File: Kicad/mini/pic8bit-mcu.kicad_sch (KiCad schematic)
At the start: 29 parts, among them IC201 TLV1117-33, IC202 MICROCHIP-PIC16F1778-ISP, K201 *Power & UART, K202 MCU 1, K203 MCU 1, K204 ICSP, K205 MCU 2, K206 MCU 2

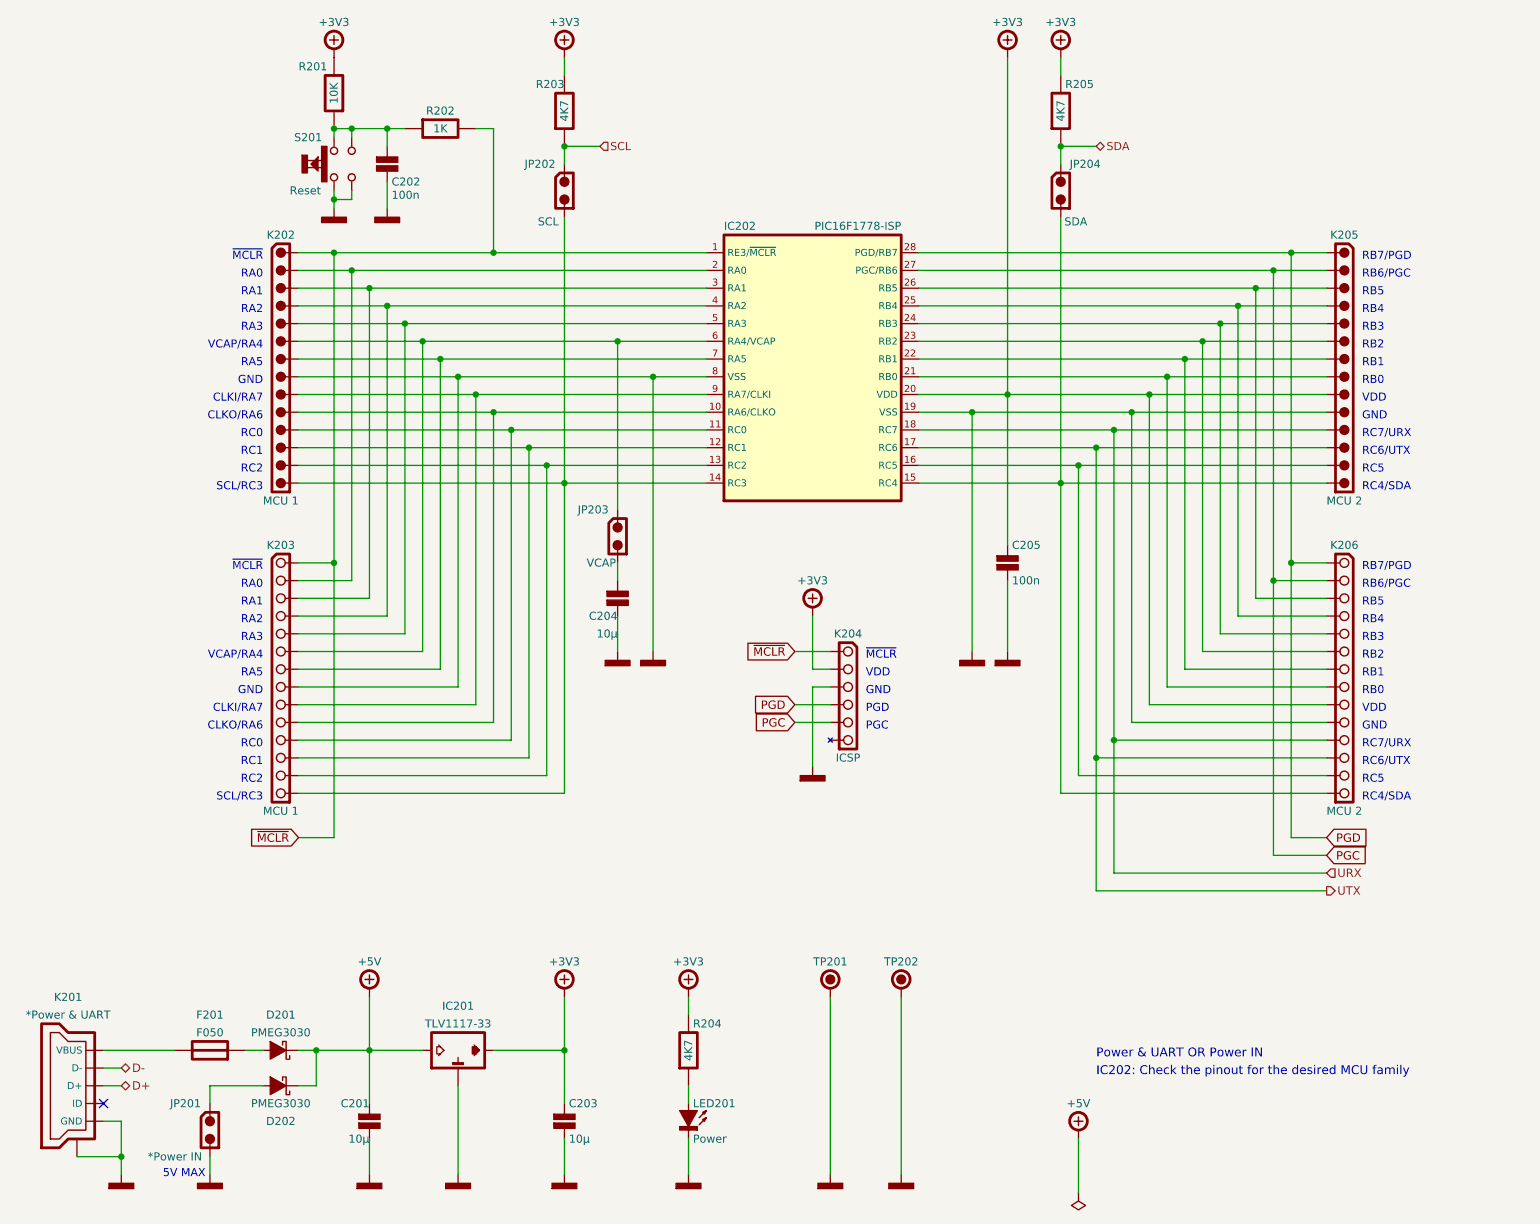
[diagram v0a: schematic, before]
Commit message: Update Mini
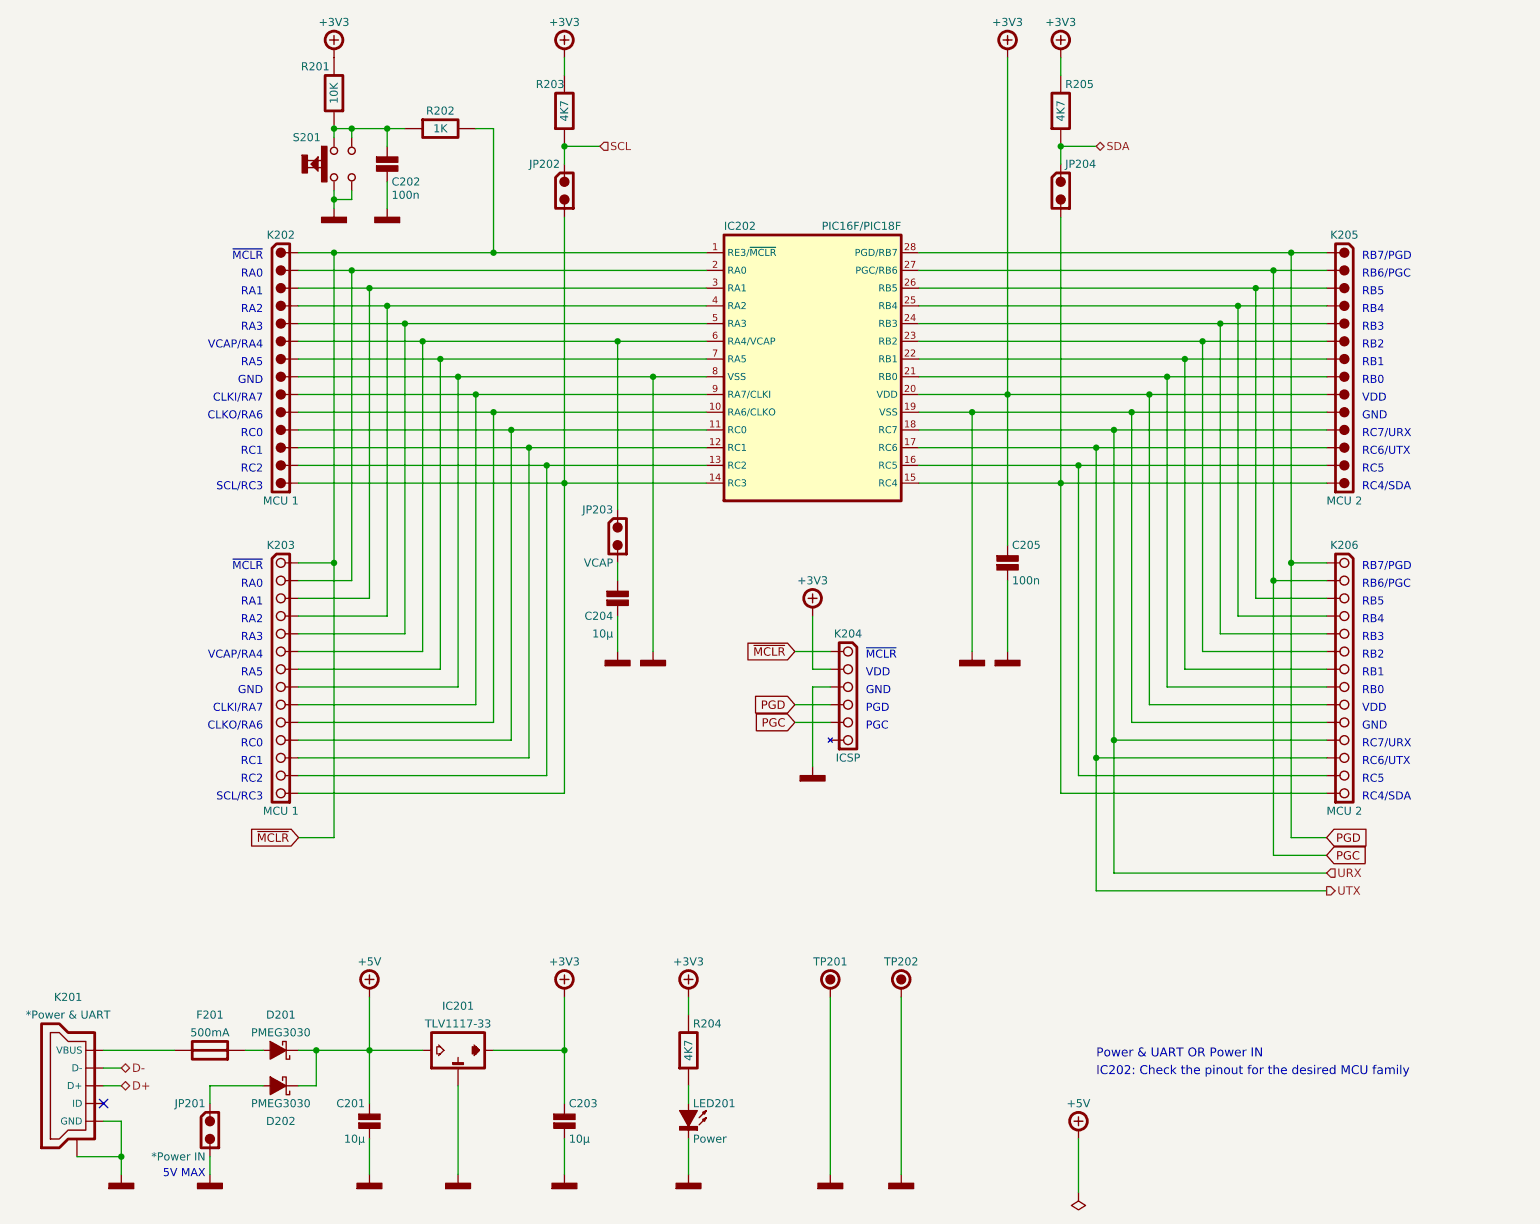
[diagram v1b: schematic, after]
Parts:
- D201, D202: symbol tronixio:PMEG3030 -> tronixio:NEXPERIA-PMEG3030; MOUSER 771-PMEG3030EP115 -> (none); Mouser (none) -> 771-PMEG3030EP115; Name (none) -> PMEG3030
- F201: value F050 -> (none); footprint tronixio:FUSE-1206 -> (none); MOUSER 652-MF-NSMF050-2 -> (none); Mouser (none) -> 652-MF-NSMF050-2; Name (none) -> 500mA
- IC201: symbol tronixio:TLV1117-33-SOT -> tronixio:TI-TLV1117-33-SOT; MOUSER 595-TLV1117-33CDC -> (none); Mouser (none) -> 595-TLV1117-33CDC; Name (none) -> TLV1117-33
- IC202: MOUSER 579-PIC16F1778-I/SP -> (none); Mouser (none) -> 579-PIC16F1778-I/SP; Name PIC16F1778-ISP -> PIC16F/PIC18F
- JP201, JP203: MOUSER 855-M20-999024 -> (none); Mouser (none) -> 855-M20-999024
- JP202: value SCL -> (none); MOUSER 855-M20-999024 -> (none); Mouser (none) -> 855-M20-999024
- JP204: value SDA -> (none); MOUSER 855-M20-999024 -> (none); Mouser (none) -> 855-M20-999024
- K201: MOUSER 649-10118193-0001LF -> (none); Mouser (none) -> 649-10118193-0001LF
- K202, K205: MOUSER 855-M20-999144 -> (none); Mouser (none) -> 855-M20-999144
- K203, K206: MOUSER 855-M20-782144 -> (none); Mouser (none) -> 855-M20-782144
- K204: MOUSER 200-SSW10602TSRA -> (none); Mouser (none) -> 200-SSW10602TSRA
- LED201: MOUSER 604-APT3216LVBCD -> (none); Mouser (none) -> 604-APT3216LVBCD
- S201: value Reset -> (none); MOUSER 688-SKRPACE010 -> (none); Mouser (none) -> 688-SKRPACE010
- TP201, TP202: MOUSER 534-5006 -> (none); Mouser (none) -> 534-5006
